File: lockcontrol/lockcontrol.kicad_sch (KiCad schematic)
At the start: 10 parts, among them J1 ButtonHeader, K1 G5Q-1A, U1 WeMos_D1_mini, U3 ULN2003, U4 Barrel_Jack_Switch, U5 Barrel_Jack_Switch

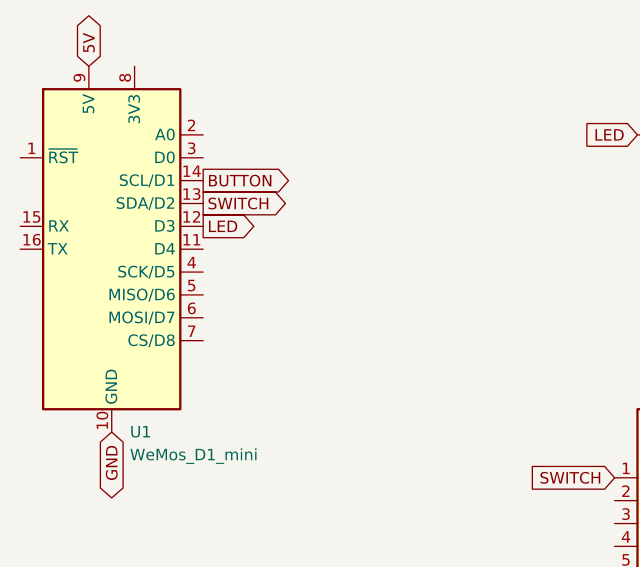
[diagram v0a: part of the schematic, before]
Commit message: capture before removing disk
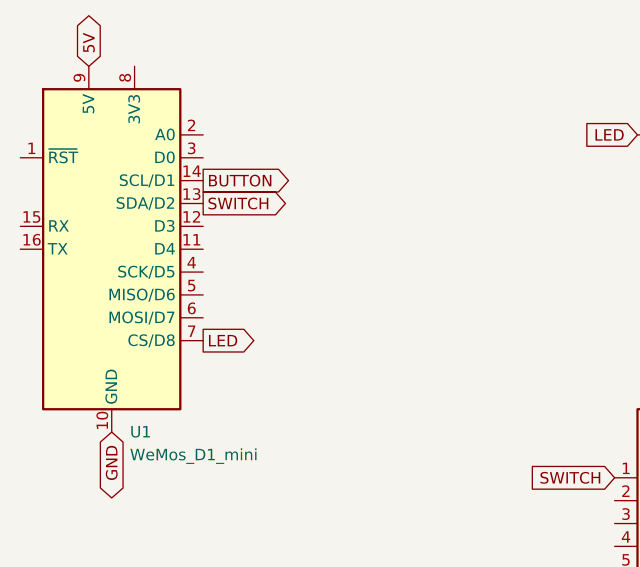
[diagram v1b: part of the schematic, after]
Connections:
- net LED: now also U1.7 (CS/D8); no longer U1.12 (D3)
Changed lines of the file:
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@@
     )
   )
-  (global_label "LED" (shape output) (at 86.36 66.04 0) (fields_autoplaced)
+  (global_label "LED" (shape output) (at 86.36 78.74 0) (fields_autoplaced)
     (effects (font (size 1.27 1.27)) (justify left))
-    (property "Intersheet References" "${INTERSHEET_REFS}" (id 0) (at 92.2202 65.9606 0)
+    (property "Intersheet References" "${INTERSHEET_REFS}" (id 0) (at 92.2202 78.6606 0)
       (effects (font (size 1.27 1.27)) (justify left) hide)
     )
